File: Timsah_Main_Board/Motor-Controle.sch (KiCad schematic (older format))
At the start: 15 parts, among them J13 SERVO Camera, J14 SAĞ ÖN, J15 SOL ÖN, J16 JSN-SR04T, J17 SAĞ ARKA, J18 SOL ARKA, J19 JSN-SR04T, J20 SERVO Gripper, J21 JSN-SR04T, J22 SAĞ ÜST, J23 SOL ÜST, J24 Power, J25 Relay Up, J26 Relay Back, U6 PCA9685PW

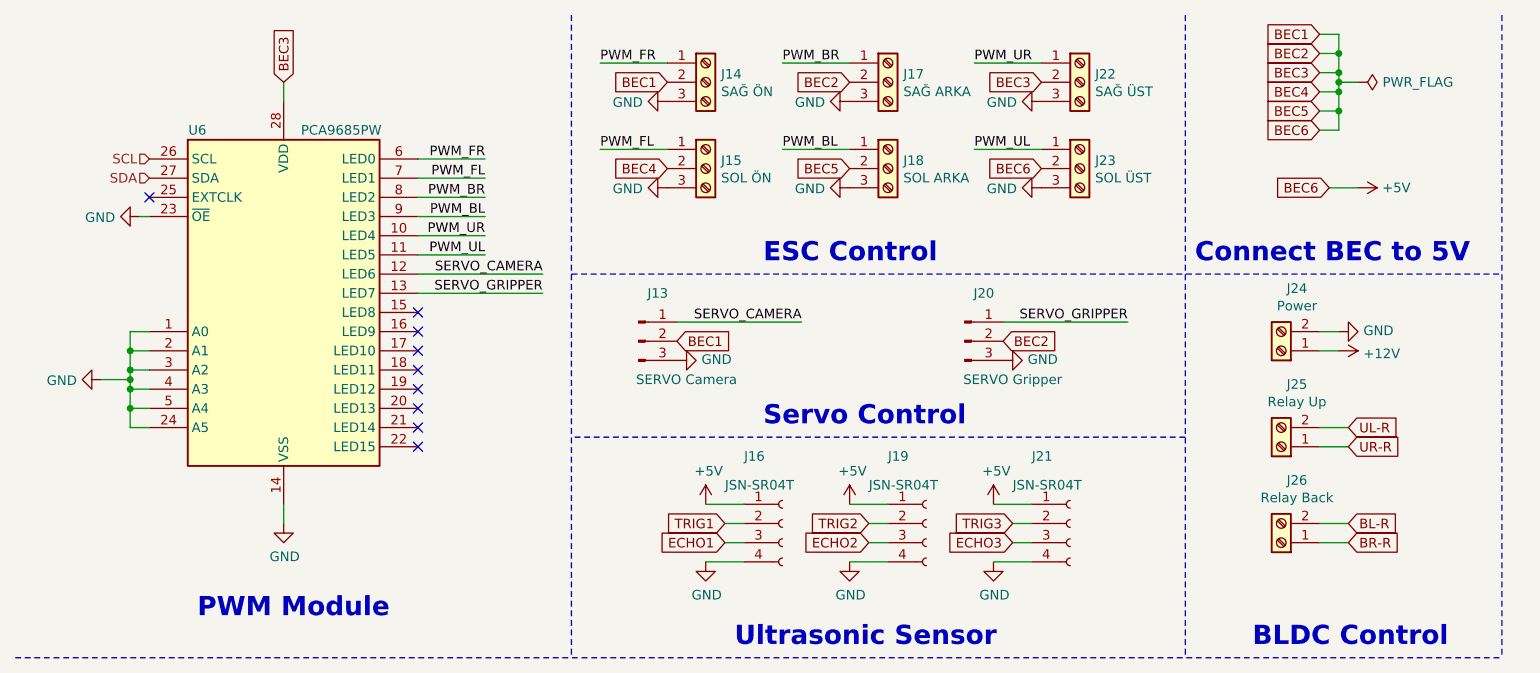
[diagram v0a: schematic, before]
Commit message: Update
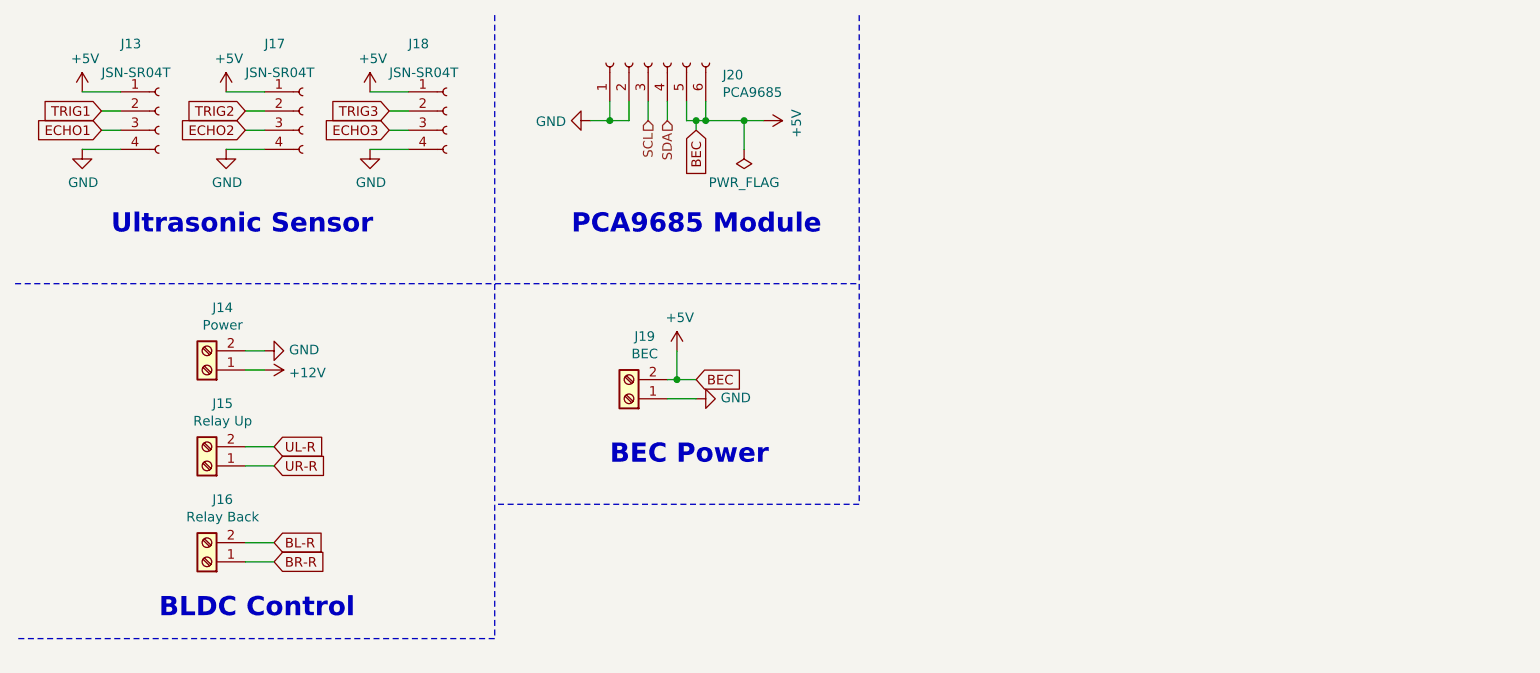
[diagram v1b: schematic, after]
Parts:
- removed J13: SERVO Camera, Connector_PinHeader_2.54mm:PinHeader_1x03_P2.54mm_Vertical, symbol Connector:Conn_01x03_Male
- removed J14: SAĞ ÖN, Connector_PinHeader_2.54mm:PinHeader_1x03_P2.54mm_Vertical, symbol Connector:Screw_Terminal_01x03
- removed J15: SOL ÖN, Connector_PinHeader_2.54mm:PinHeader_1x03_P2.54mm_Vertical, symbol Connector:Screw_Terminal_01x03
- removed J17: SAĞ ARKA, Connector_PinHeader_2.54mm:PinHeader_1x03_P2.54mm_Vertical, symbol Connector:Screw_Terminal_01x03
- removed J18: SOL ARKA, Connector_PinHeader_2.54mm:PinHeader_1x03_P2.54mm_Vertical, symbol Connector:Screw_Terminal_01x03
- removed J20: SERVO Gripper, Connector_PinHeader_2.54mm:PinHeader_1x03_P2.54mm_Vertical, symbol Connector:Conn_01x03_Male
- removed J22: SAĞ ÜST, Connector_PinHeader_2.54mm:PinHeader_1x03_P2.54mm_Vertical, symbol Connector:Screw_Terminal_01x03
- removed J23: SOL ÜST, Connector_PinHeader_2.54mm:PinHeader_1x03_P2.54mm_Vertical, symbol Connector:Screw_Terminal_01x03
- removed U6: PCA9685PW, Package_SO:TSSOP-28_4.4x9.7mm_P0.65mm, symbol Driver_LED:PCA9685PW
- added J19: BEC, TerminalBlock_4Ucon:TerminalBlock_4Ucon_1x02_P3.50mm_Vertical, symbol Connector:Screw_Terminal_01x02
- added J20: PCA9685, Connector_PinSocket_2.54mm:PinSocket_1x06_P2.54mm_Vertical, symbol Connector:Conn_01x06_Female
- renumbered J16 to J13, J24 to J14, J25 to J15, J26 to J16, J19 to J17, J21 to J18
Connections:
- net +5V: now also J19.2 (Pin_2), J20.5 (Pin_5), J20.6 (Pin_6)
- net GND: now also J19.1 (Pin_1), J20.1 (Pin_1), J20.2 (Pin_2)
- net SCL: now also J20.3 (Pin_3)
- net SDA: now also J20.4 (Pin_4)
- no-connect marks 9 -> 0
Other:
- note added: "BEC Power"
- note added: "PCA9685 Module"
- note removed: "Connect BEC to 5V"
- note removed: "ESC Control"
- note removed: "PWM Module"
- note removed: "Servo Control"
- moved on the sheet: J13, J14, J15, J16, J17, J18
